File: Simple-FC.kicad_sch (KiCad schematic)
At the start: 55 parts, among them J1 USB_C_Receptacle_USB2.0_14P, J2 Micro_SD_Card, SW1 SW_Push, U1 RP2350A, U2 MMC5983MA, U3 LSM6DSM, U4 BMP384, U5 TPS631000, U6 W25Q128JVS, Y1 ABM8-272-T3

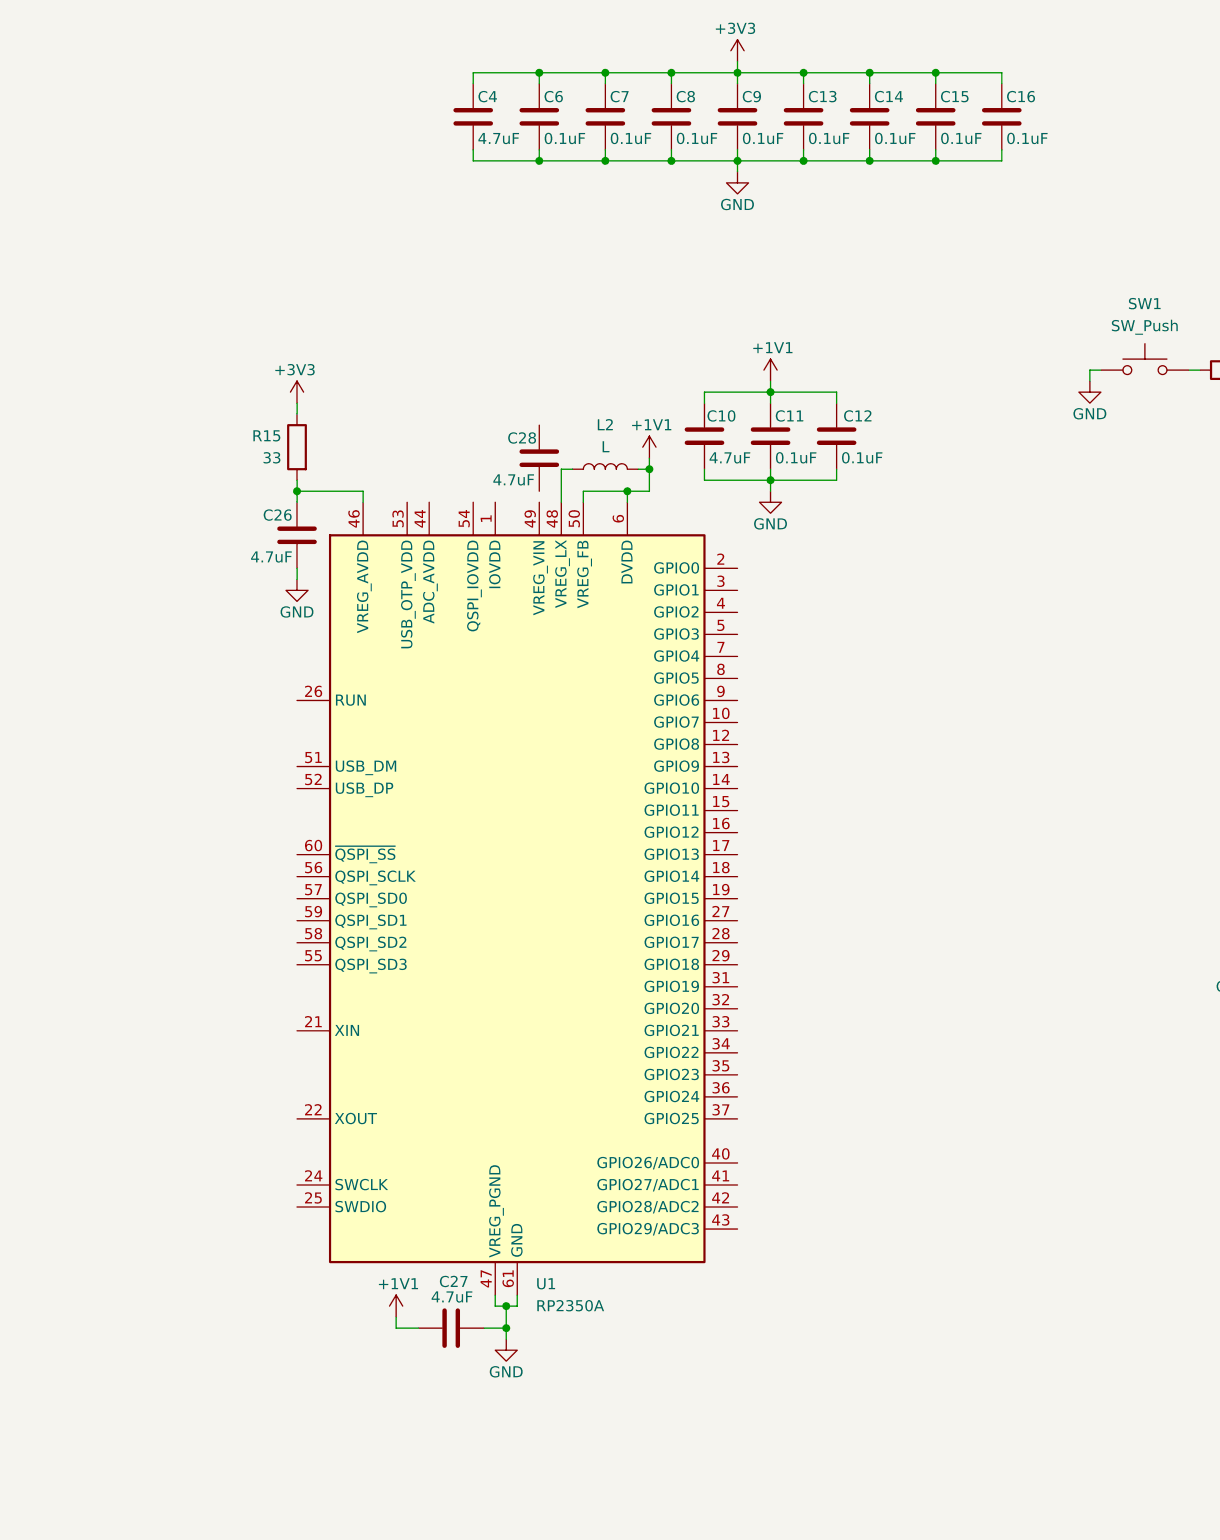
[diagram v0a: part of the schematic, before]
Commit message: finished mcu power circuit
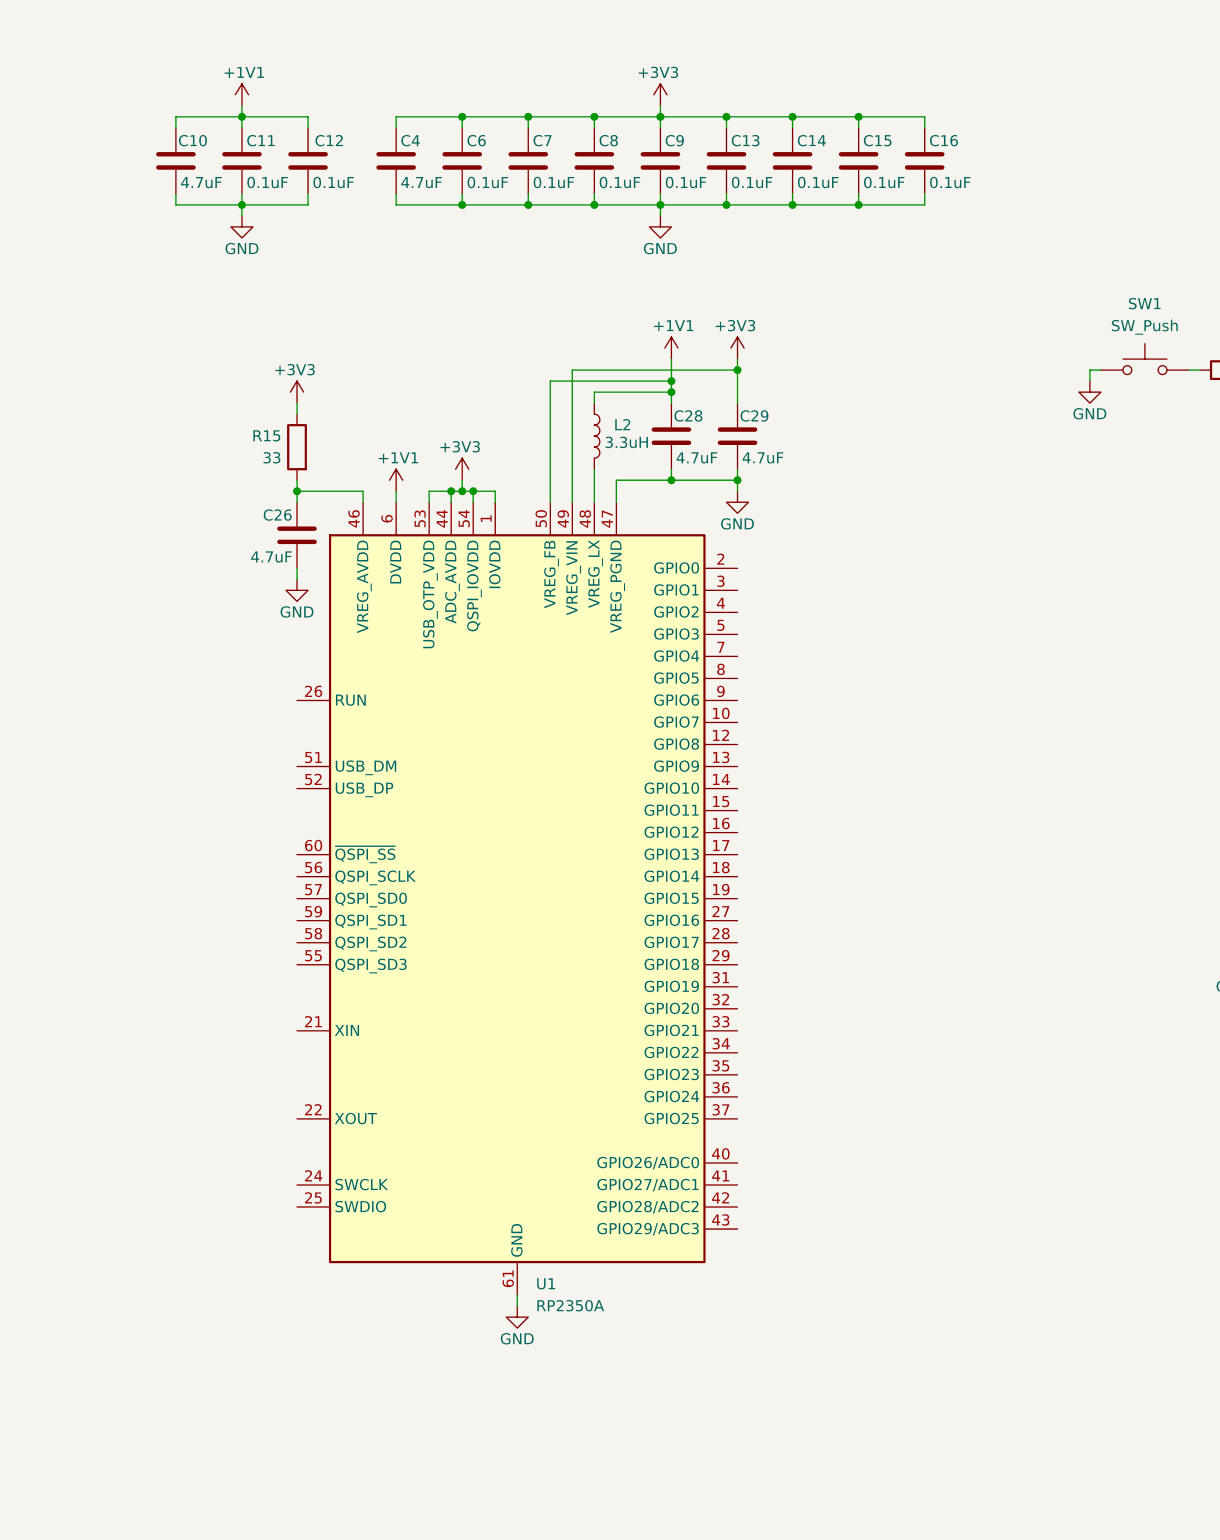
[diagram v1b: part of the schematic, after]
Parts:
- removed C27: 4.7uF, Capacitor_SMD:C_0402_1005Metric, symbol Device:C
- added C29: 4.7uF, Capacitor_SMD:C_0402_1005Metric, symbol Device:C
- L2: value L -> 3.3uH
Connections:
- net +1V1: now also C28.1, L2.1; no longer L2.2
- net +3V3: now also U1.1 (IOVDD), U1.11 (IOVDD), U1.20 (IOVDD), U1.30 (IOVDD), U1.38 (IOVDD), U1.44 (ADC_AVDD), U1.45 (IOVDD), U1.49 (VREG_VIN), U1.53 (USB_OTP_VDD), U1.54 (QSPI_IOVDD), C29.1
- net GND: now also C28.2, C29.2
- net at U1.48 (VREG_LX): now also L2.2; no longer L2.1
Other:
- moved on the sheet: C10, C11, C12, C13, C14, C15, C16, C4, C6, C7, C8, C9
